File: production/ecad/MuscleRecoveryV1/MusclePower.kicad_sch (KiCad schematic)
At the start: 23 parts, among them IC1 LC709203FQH-01TWG, Q1 FDN340P, U1 AP1117-33, U2 MCP73831-2-OT

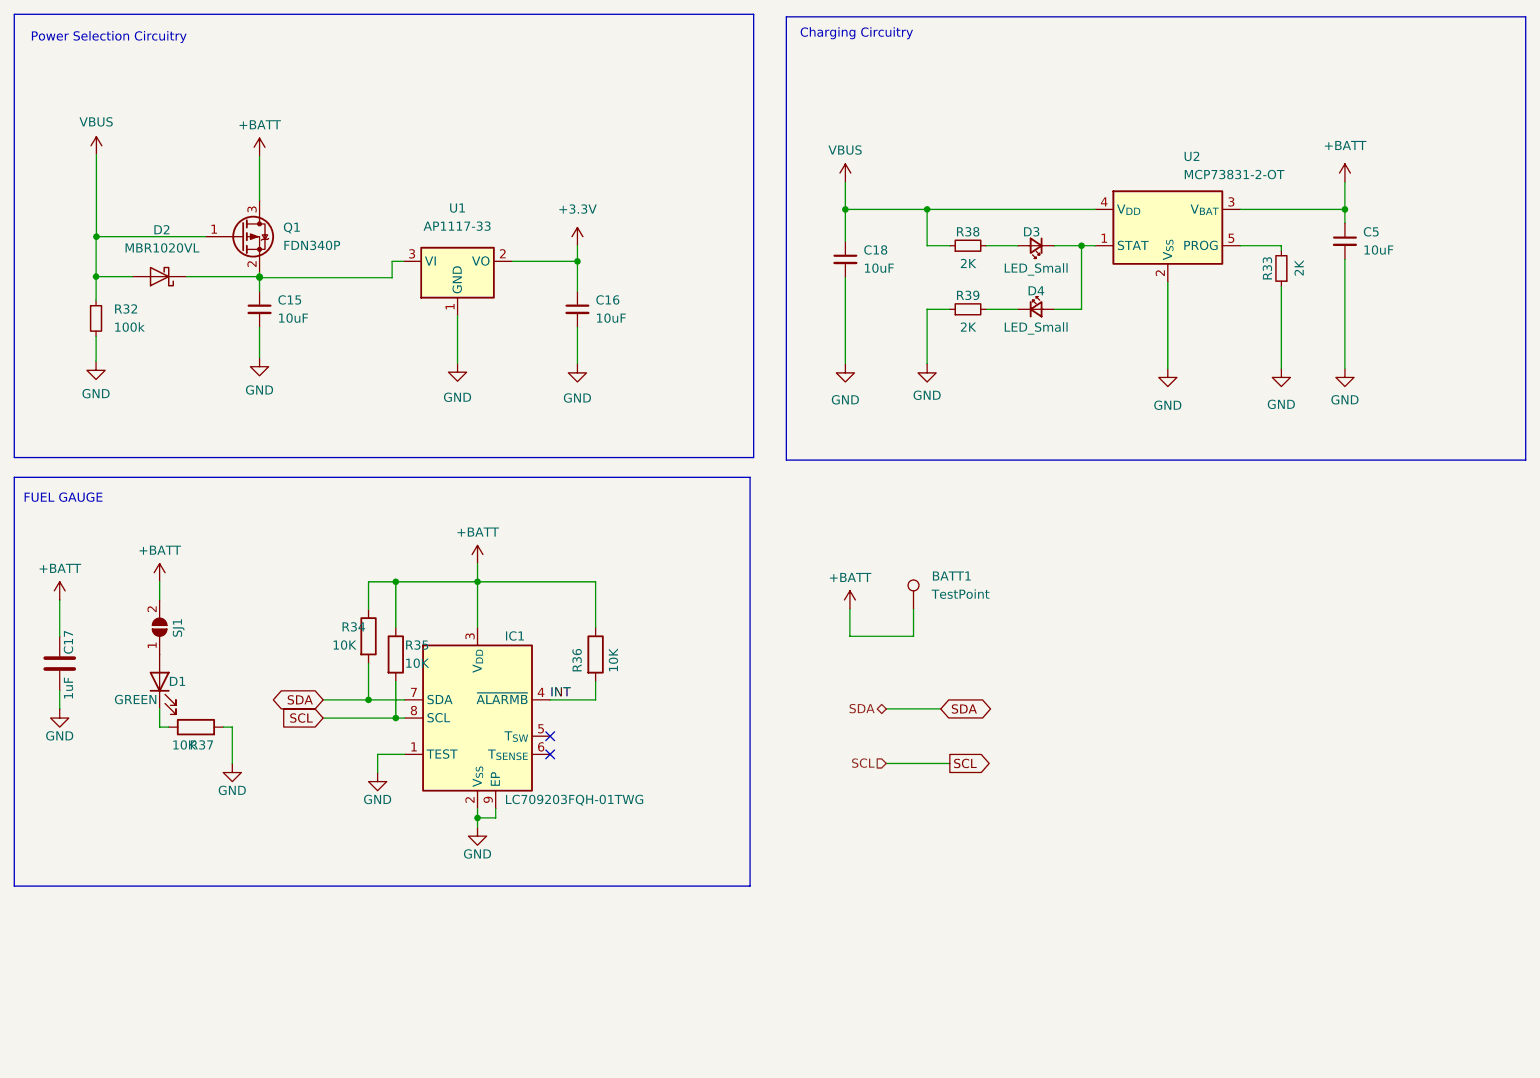
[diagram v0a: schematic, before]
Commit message: Display commit 1
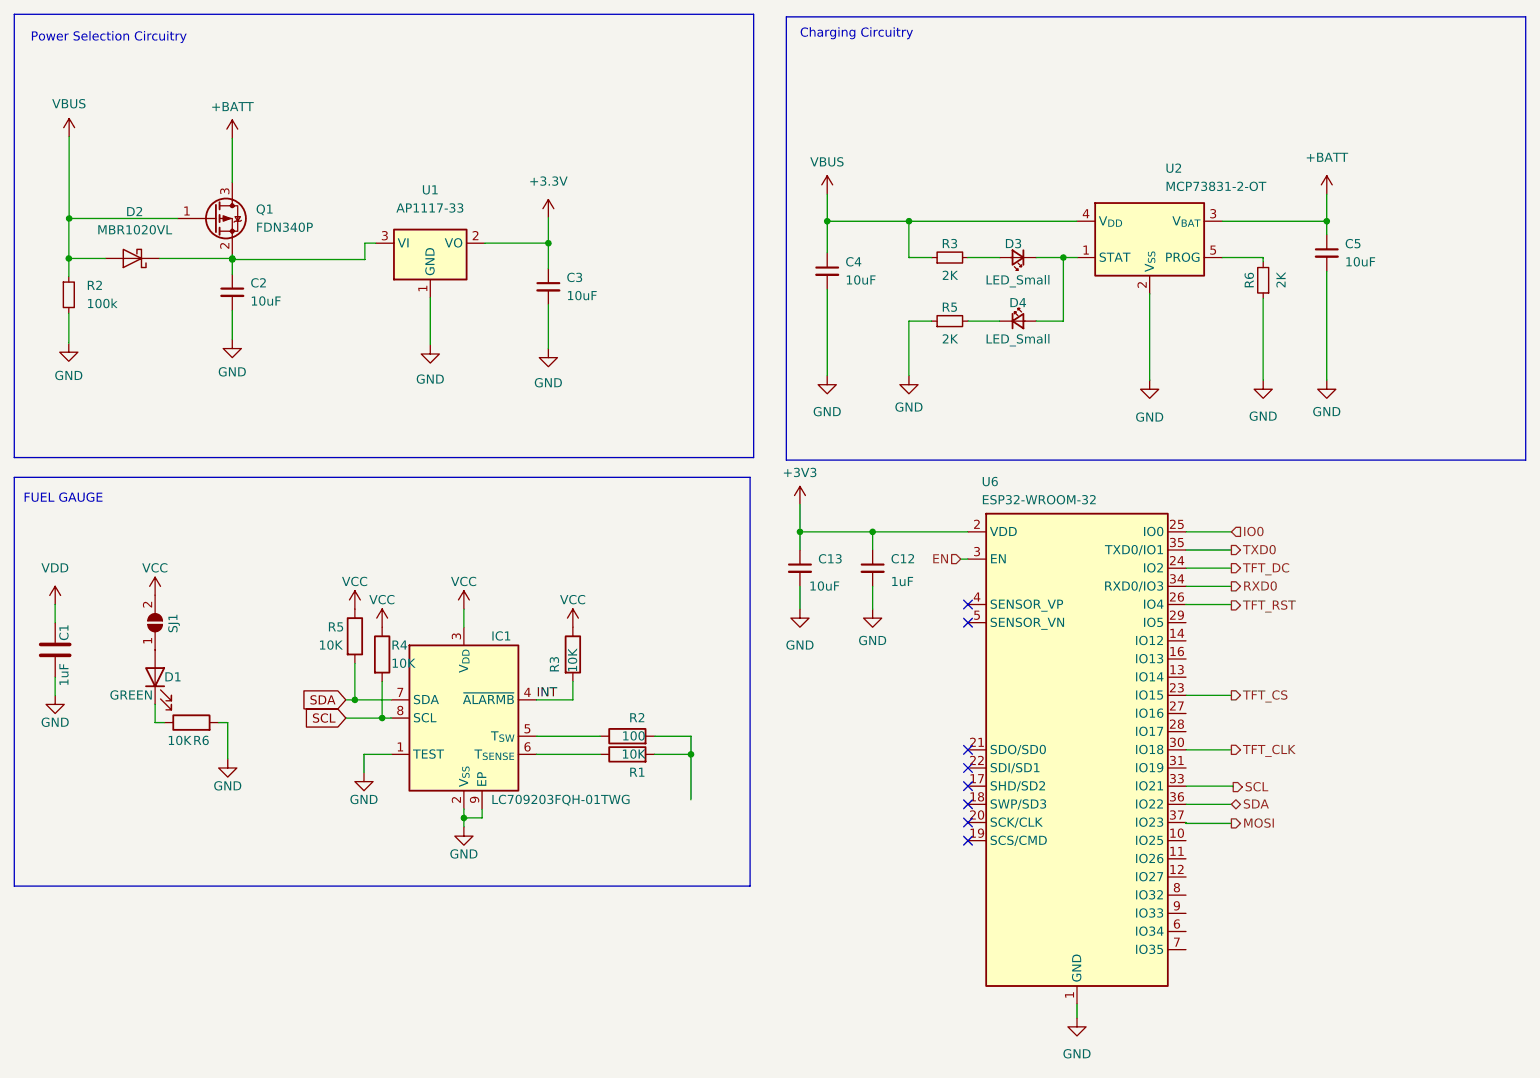
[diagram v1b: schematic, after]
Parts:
- removed BATT1: TestPoint, symbol Connector:TestPoint
- removed C15, C16, C18: 10uF, symbol Device:C_Small
- removed C17: 1uF, symbol Device:C
- removed R32: 100k, symbol Device:R_Small
- removed R33, R38, R39: 2K, symbol Device:R_Small
- removed R34, R35, R37: 10K, symbol Device:R
- removed R36: 10K, Resistor_SMD:R_0805_2012Metric, symbol Device:R
- added C1: 1uF, symbol Device:C
- added C12: 1uF, symbol Device:C_Small
- added C13, C2, C3, C4: 10uF, symbol Device:C_Small
- added R1, R3: 10K, Resistor_SMD:R_0805_2012Metric, symbol Device:R
- added R2: 100, Resistor_SMD:R_0805_2012Metric, symbol Device:R
- added R2: 100k, symbol Device:R_Small
- added R3, R5, R6: 2K, symbol Device:R_Small
- added R4, R5, R6: 10K, symbol Device:R
- added U6: ESP32-WROOM-32, RF_Module:ESP32-WROOM-32, symbol RF_Module:ESP32-WROOM-32
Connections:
- net +3.3V: now also C3.1
- net +BATT: no longer IC1.3 (V_{DD}), SJ1.2 (B)
- net GND: now also C1.2, C12.2, C13.2, C2.2, C3.2, C4.2, R2.2, R5.1, R6.1, R6.2, U6.1 (GND), U6.15 (GND), U6.38 (GND), U6.39 (GND)
- net INT: now also R3.2
- net SCL: now also R4.2, U6.33 (IO21)
- net SDA: now also R5.2, U6.36 (IO22)
- net VBUS: now also C4.1, R2.1, R3.1
- net at D3.2 (A): now also R3.2
- net at IC1.5 (T_{SW}): now also R2.1
- net at IC1.6 (T_{SENSE}): now also R1.1
- net at D2.1 (K), Q1.2 (S), U1.3 (VI): now also C2.1
- net at D4.1 (K): now also R5.2
- net at D1.1 (K): now also R6.1
- net at U2.5 (PROG): now also R6.2
- new net: R1.2, R2.2
- new net +3V3: C12.1, C13.1, U6.2 (VDD)
- new net EN: U6.3 (EN)
- new net IO0: U6.25 (IO0)
- new net MOSI: U6.37 (IO23)
- new net RXD0: U6.34 (RXD0/IO3)
- new net TFT_CLK: U6.30 (IO18)
- new net TFT_CS: U6.23 (IO15)
- new net TFT_DC: U6.24 (IO2)
- new net TFT_RST: U6.26 (IO4)
- new net TXD0: U6.35 (TXD0/IO1)
- new net VCC: IC1.3 (V_{DD}), R3.1, R4.1, R5.1, SJ1.2 (B)
- new net VDD: C1.1
- no-connect marks 2 -> 8
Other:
- moved on the sheet: D1, D2, D3, D4, IC1, Q1, SJ1, U1, U2
